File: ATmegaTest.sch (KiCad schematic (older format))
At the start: 16 parts, among them P1 Digital, P10 CONN_01X01, P11 CONN_01X01, P12 CONN_01X01, P13 CONN_01X01, P2 Power, P3 Analog, P4 Analog, P5 PWM, P6 PWM, P7 Communication, P8 CONN_01X01, P9 CONN_01X01, SW1 SW_DIP_x01

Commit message: Update ATmegaTest.sch
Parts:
- SW1: footprint Button_Switch_SMD:SW_SPST_CK_KXT3 -> (none)
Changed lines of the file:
@@
 F 0 "SW1" H 7240 2227 50  0000 C CNN
 F 1 "SW_DIP_x01" H 7240 2136 50  0000 C CNN
-F 2 "Button_Switch_SMD:SW_SPST_CK_KXT3" H 7240 1960 50  0001 C CNN
+F 2 "" H 7240 1960 50  0001 C CNN
 F 3 "~" H 7240 1960 50  0001 C CNN
 	1    7240 1960
@@
 Reset
 $Comp
-L power:GND #PWR?
+L power:GND #PWR0101
 U 1 1 5DB848D9
 P 6750 1920
-F 0 "#PWR?" H 6750 1670 50  0001 C CNN
+F 0 "#PWR0101" H 6750 1670 50  0001 C CNN
 F 1 "GND" H 6750 1770 50  0000 C CNN
 F 2 "" H 6750 1920 50  0000 C CNN

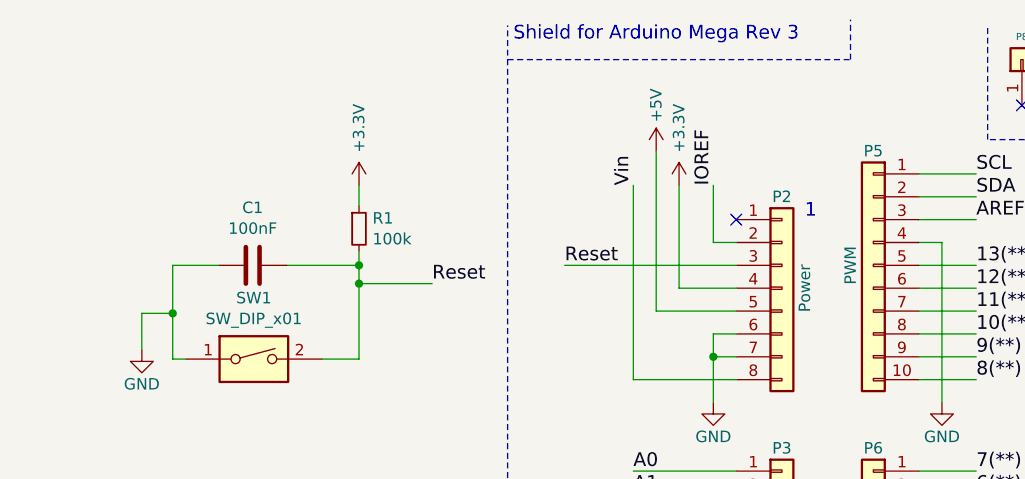
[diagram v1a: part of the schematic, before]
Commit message: DividerCkt
Voltage Divider with analogInput  to ATMEGA
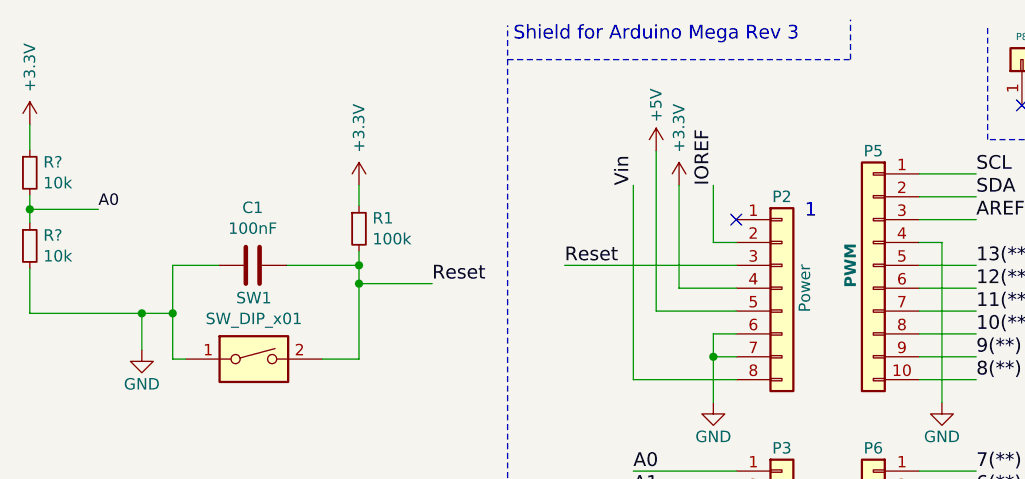
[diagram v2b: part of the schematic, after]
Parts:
- added R? (x2): 10k, Resistor_SMD:R_0603_1608Metric, symbol Device:R_Small
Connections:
- net +3V3: now also R?.1
- net A0: now also R?.1, R?.2
- net GND: now also R?.2
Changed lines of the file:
@@
 EESchema Schematic File Version 4
-LIBS:ATmegaTest-cache
 EELAYER 29 0
 EELAYER END
@@
 P 9950 1550
 F 0 "P5" H 9950 2050 50  0000 C CNN
-F 1 "PWM" V 10050 1550 50  0000 C CNN
+F 1 "PWM" V 10050 1550 50  0000 C CNB
 F 2 "Socket_Arduino_Mega:Socket_Strip_Arduino_1x10" H 9950 1550 50  0001 C CNN
 F 3 "" H 9950 1550 50  0000 C CNN
@@
 	1    0    0    -1
 $EndComp
+$Comp
+L power:+3V3 #PWR?
+U 1 1 5DB90B5B
+P 6260 935
+F 0 "#PWR?" H 6260 785 50  0001 C CNN
+F 1 "+3.3V" V 6260 1185 50  0000 C CNN
+F 2 "" H 6260 935 50  0000 C CNN
+F 3 "" H 6260 935 50  0000 C CNN
+	1    6260 935
+	1    0    0    -1
+$EndComp
+$Comp
+L Device:R_Small R?
+U 1 1 5DB97808
+P 6260 1145
+F 0 "R?" H 6319 1191 50  0000 L CNN
+F 1 "10k" H 6319 1100 50  0000 L CNN
+F 2 "Resistor_SMD:R_0603_1608Metric" H 6260 1145 50  0001 C CNN
+F 3 "~" H 6260 1145 50  0001 C CNN
+	1    6260 1145
+	1    0    0    -1
+$EndComp
+Wire Wire Line
+	6260 1245 6260 1305
+Wire Wire Line
+	6260 1045 6260 935
+Wire Wire Line
+	6260 1760 6750 1760
+Connection ~ 6750 1760
+$Comp
+L Device:R_Small R?
+U 1 1 5DBA2C8F
+P 6260 1465
+F 0 "R?" H 6319 1511 50  0000 L CNN
+F 1 "10k" H 6319 1420 50  0000 L CNN
+F 2 "Resistor_SMD:R_0603_1608Metric" H 6260 1465 50  0001 C CNN
+F 3 "~" H 6260 1465 50  0001 C CNN
+	1    6260 1465
+	1    0    0    -1
+$EndComp
+Wire Wire Line
+	6260 1565 6260 1760
+Wire Wire Line
+	6260 1305 6560 1305
+Connection ~ 6260 1305
+Wire Wire Line
+	6260 1305 6260 1365
+Text Label 6560 1305 0    50   ~ 0
+A0
 $EndSCHEMATC

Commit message: Revert "DividerCkt"
This reverts commit 058e6e4fb967e27780ca64c39ae31b78ca90827e.
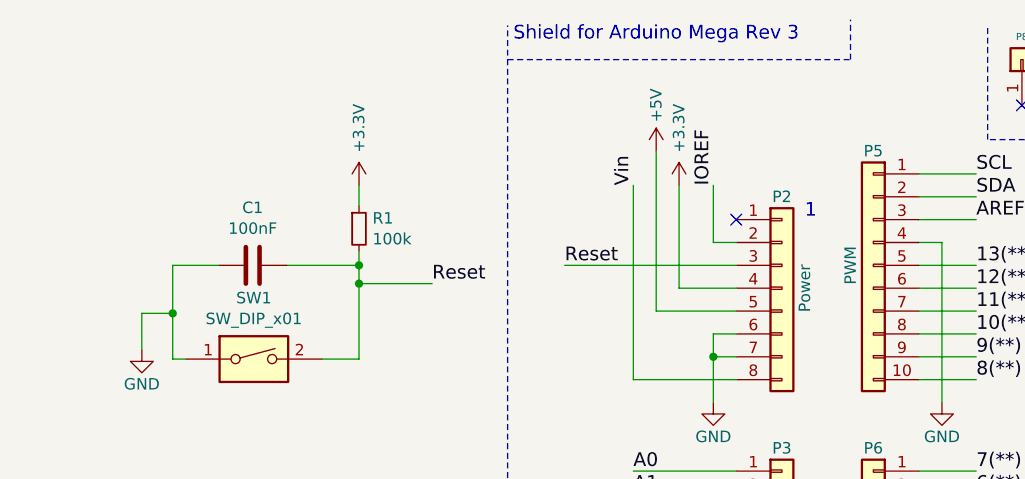
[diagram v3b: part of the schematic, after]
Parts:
- removed R? (x2): 10k, Resistor_SMD:R_0603_1608Metric, symbol Device:R_Small
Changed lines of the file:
@@
 EESchema Schematic File Version 4
+LIBS:ATmegaTest-cache
 EELAYER 29 0
 EELAYER END
@@
 P 9950 1550
 F 0 "P5" H 9950 2050 50  0000 C CNN
-F 1 "PWM" V 10050 1550 50  0000 C CNB
+F 1 "PWM" V 10050 1550 50  0000 C CNN
 F 2 "Socket_Arduino_Mega:Socket_Strip_Arduino_1x10" H 9950 1550 50  0001 C CNN
 F 3 "" H 9950 1550 50  0000 C CNN
@@
 	1    0    0    -1
 $EndComp
-$Comp
-L power:+3V3 #PWR?
-U 1 1 5DB90B5B
-P 6260 935
-F 0 "#PWR?" H 6260 785 50  0001 C CNN
-F 1 "+3.3V" V 6260 1185 50  0000 C CNN
-F 2 "" H 6260 935 50  0000 C CNN
-F 3 "" H 6260 935 50  0000 C CNN
-	1    6260 935
-	1    0    0    -1
-$EndComp
-$Comp
-L Device:R_Small R?
-U 1 1 5DB97808
-P 6260 1145
-F 0 "R?" H 6319 1191 50  0000 L CNN
-F 1 "10k" H 6319 1100 50  0000 L CNN
-F 2 "Resistor_SMD:R_0603_1608Metric" H 6260 1145 50  0001 C CNN
-F 3 "~" H 6260 1145 50  0001 C CNN
-	1    6260 1145
-	1    0    0    -1
-$EndComp
-Wire Wire Line
-	6260 1245 6260 1305
-Wire Wire Line
-	6260 1045 6260 935
-Wire Wire Line
-	6260 1760 6750 1760
-Connection ~ 6750 1760
-$Comp
-L Device:R_Small R?
-U 1 1 5DBA2C8F
-P 6260 1465
-F 0 "R?" H 6319 1511 50  0000 L CNN
-F 1 "10k" H 6319 1420 50  0000 L CNN
-F 2 "Resistor_SMD:R_0603_1608Metric" H 6260 1465 50  0001 C CNN
-F 3 "~" H 6260 1465 50  0001 C CNN
-	1    6260 1465
-	1    0    0    -1
-$EndComp
-Wire Wire Line
-	6260 1565 6260 1760
-Wire Wire Line
-	6260 1305 6560 1305
-Connection ~ 6260 1305
-Wire Wire Line
-	6260 1305 6260 1365
-Text Label 6560 1305 0    50   ~ 0
-A0
 $EndSCHEMATC
